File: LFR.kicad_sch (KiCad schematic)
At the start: 52 parts, among them J1 USB_B_Micro, J2 Conn_01x04_Pin, SW1 SW_Push, U1 STM32F103C8Tx, U2 DM-OLED096-636, U3 TB6612FNG, U4 MP1584EN, U5 MP1584EN, Y1 8MHz

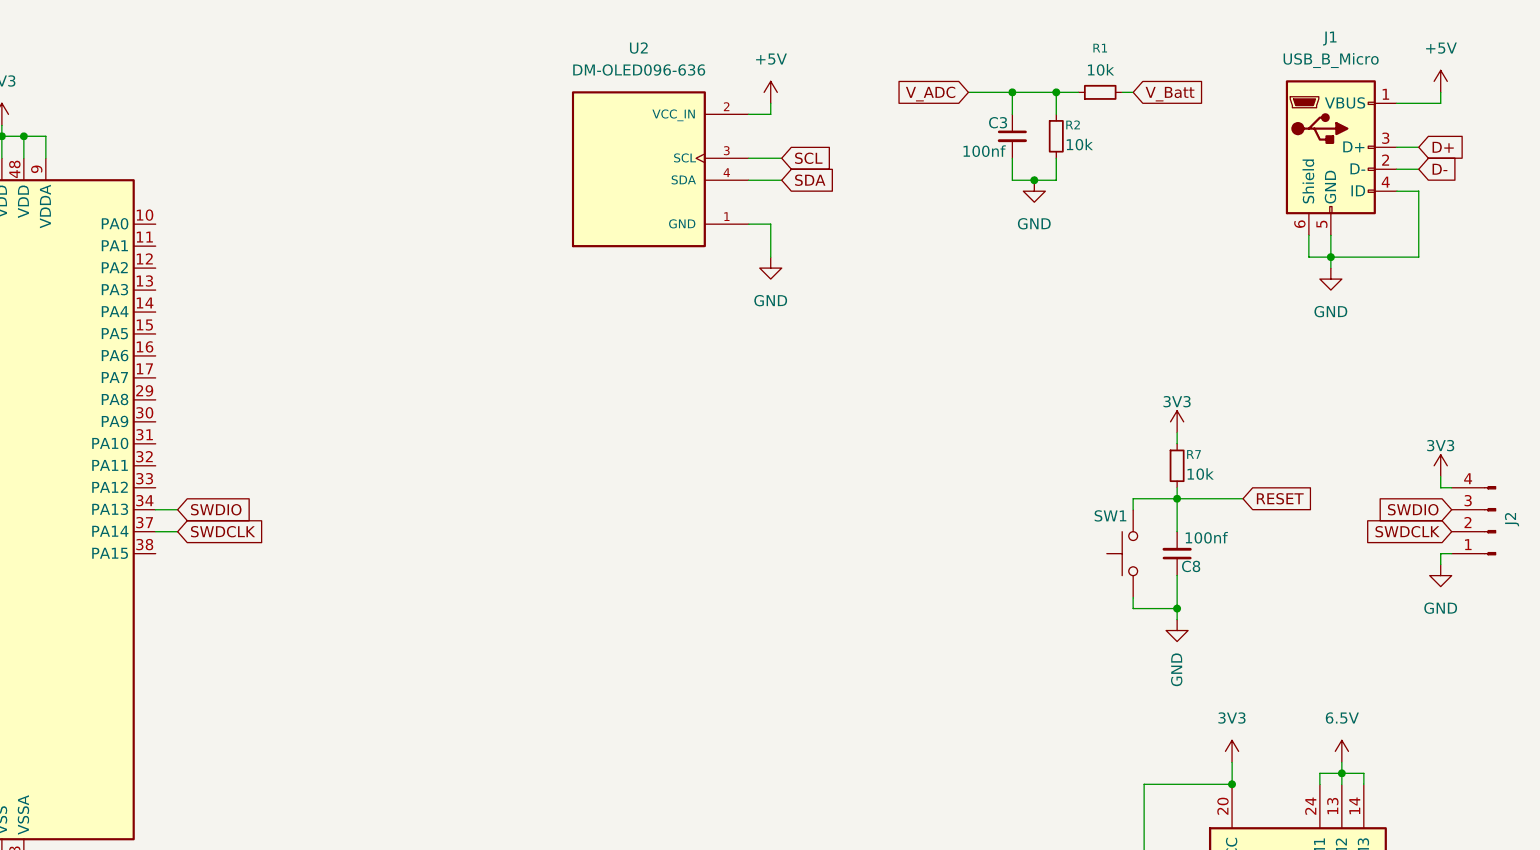
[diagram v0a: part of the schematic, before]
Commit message: save
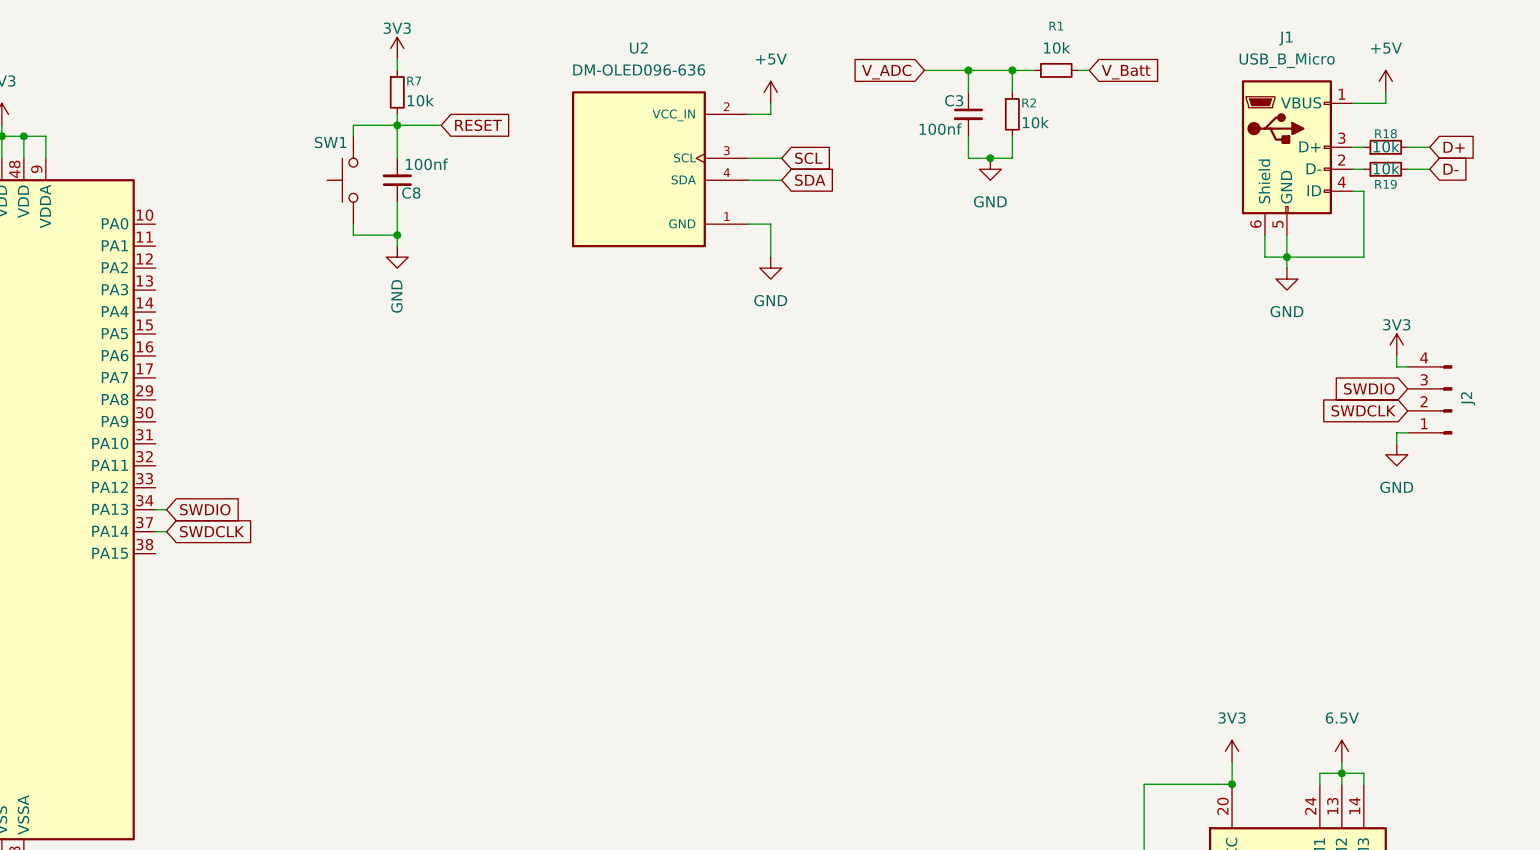
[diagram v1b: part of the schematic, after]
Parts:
- added R18, R19: 10k, symbol Device:R_Small
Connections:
- net D+: now also R18.2; no longer J1.3 (D+)
- net D-: now also R19.2; no longer J1.2 (D-)
- new net: J1.2 (D-), R19.1
- new net: J1.3 (D+), R18.1
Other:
- moved on the sheet: C3, C8, J1, J2, R1, R2, R7, SW1
